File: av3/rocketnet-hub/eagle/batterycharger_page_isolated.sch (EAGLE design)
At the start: 45 parts, among them Q1 SIS412DNSOP-8, Q2 FDS6680ASOIC-8, Q3 FDS6680ASOIC-8, Q4 BSS138W-7-F, Q5 FDS6680ASOIC-8, Q6 SIS412DNSOP-8, U1 BQ24725QFN-20, U8 4.7uH

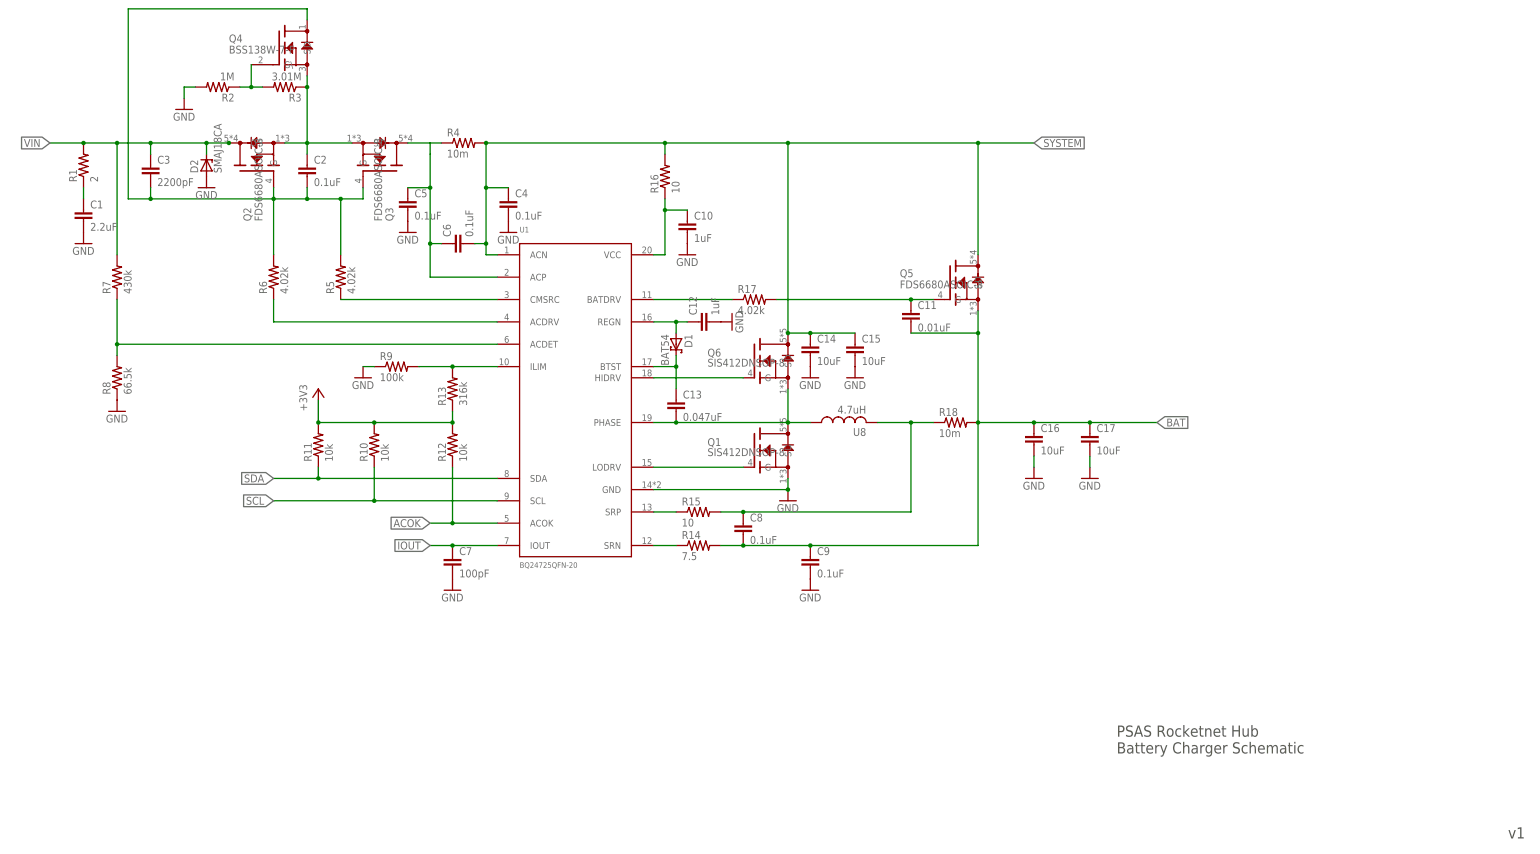
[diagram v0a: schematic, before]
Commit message: battery charger current state
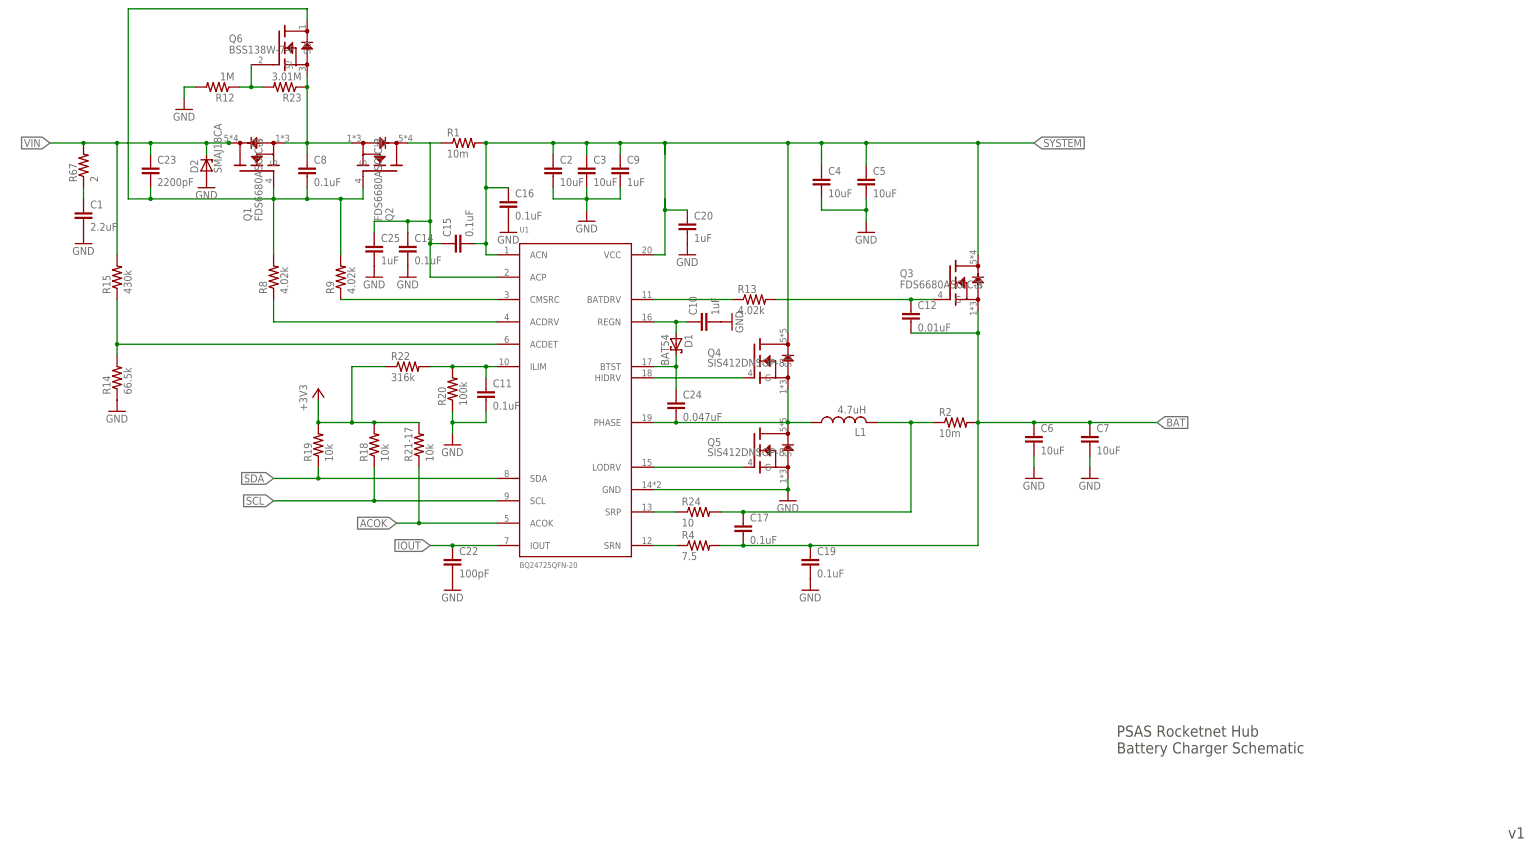
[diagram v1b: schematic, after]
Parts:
- removed C13: 0.047uF, rcl_custom:C-EU0603-B
- removed R10, R11: 10k, rcl_custom:R-US_R0603
- removed R16: 10, rcl_custom:R-US_1206-B
- removed R17, R5, R6: 4.02k, rcl_custom:R-US_0603-B
- removed R3: 3.01M, rcl_custom:R-US_0603-B
- removed R7: 430k, rcl_custom:R-US_0603-B
- added C19: 0.1uF, rcl_custom:C-EU0402-B
- added C20, C25: 1uF, rcl_custom:C-EU0603-B
- added C22: 100pF, rcl_custom:C-EU0402-B
- added C23: 2200pF, rcl_custom:C-EU0402-B
- added C24: 0.047uF, rcl_custom:C-EU0402-B
- added R19, R21-17: 10k, rcl_custom:R-US_0402-B
- added R20: 100k, rcl_custom:R-US_0402-B
- added R22: 316k, rcl_custom:R-US_0402-B
- added R23: 3.01M, rcl_custom:R-US_0402-B
- added R24: 10, rcl_custom:R-US_0603-B
- added R67: 2, rcl_custom:R-US_1206-B
- C11: value 0.01uF -> 0.1uF; device rcl_custom:C-EU0603-B -> rcl_custom:C-EU0402-B
- C12: value 1uF -> 0.01uF; device rcl_custom:C-EU0603-B -> rcl_custom:C-EU0402-B
- C14, C15, C16, C17: value 10uF -> 0.1uF; device rcl_custom:C-EU1206-B -> rcl_custom:C-EU0402-B
- C2, C4, C5, C6: value 0.1uF -> 10uF; device rcl_custom:C-EU0603-B -> rcl_custom:C-EU1206-B
- C3: value 2200pF -> 10uF; device rcl_custom:C-EU0603-B -> rcl_custom:C-EU1206-B
- C7: value 100pF -> 10uF; device rcl_custom:C-EUC0603 -> rcl_custom:C-EU1206-B
- C8: device rcl_custom:C-EU0603-B -> rcl_custom:C-EU0402-B
- C9: value 0.1uF -> 1uF
- Q1: value SIS412DNSOP-8 -> FDS6680ASOIC-8; device RNH_SIS412DN:SIS412DNSOP-8 -> RNH_FDS6680A:FDS6680ASOIC-8
- Q4: value BSS138W-7-F -> SIS412DNSOP-8; device RNH_BSS138W-7-F:BSS138W-7-F -> RNH_SIS412DN:SIS412DNSOP-8
- Q5: value FDS6680ASOIC-8 -> SIS412DNSOP-8; device RNH_FDS6680A:FDS6680ASOIC-8 -> RNH_SIS412DN:SIS412DNSOP-8
- Q6: value SIS412DNSOP-8 -> BSS138W-7-F; device RNH_SIS412DN:SIS412DNSOP-8 -> RNH_BSS138W-7-F:BSS138W-7-F
- R1: value 2 -> 10m
- R12: value 10k -> 1M; device rcl_custom:R-US_R0603 -> rcl_custom:R-US_0402-B
- R13: value 316k -> 4.02k; device rcl_custom:R-US_R0603 -> rcl_custom:R-US_0402-B
- R14: value 7.5 -> 66.5k; device rcl_custom:R-US_0603-B -> rcl_custom:R-US_0402-B
- R15: value 10 -> 430k; device rcl_custom:R-US_0603-B -> rcl_custom:R-US_0402-B
- R18: value 10m -> 10k; device rcl_custom:R-US_1206-B -> rcl_custom:R-US_0402-B
- R2: value 1M -> 10m; device rcl_custom:R-US_0603-B -> rcl_custom:R-US_1206-B
- R4: value 10m -> 7.5; device rcl_custom:R-US_1206-B -> rcl_custom:R-US_0603-B
- R8: value 66.5k -> 4.02k; device rcl_custom:R-US_1206-B -> rcl_custom:R-US_0402-B
- R9: value 100k -> 4.02k; device rcl_custom:R-US_R0603 -> rcl_custom:R-US_0402-B
- renumbered U8 to L1
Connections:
- removed net N$17: C10.1, R16.1, U1.VCC
- net +3V3: now also R18.2, R19.2, R21-17.2, R22.1; no longer R10.2, R11.2, R12.2, R13.1
- net ACOK: now also R21-17.1; no longer R12.1
- net BAT: now also C12.2, C17.2, C19.1, C6.1, C7.1, Q3.S, R2.2, R4.2; no longer C11.2, C16.1, C17.1, C8.2, C9.1, Q5.S, R14.2, R18.2
- net GND: now also C11.2, C19.2, C2.2, C20.2, C22.2, C25.2, C3.2, C6.2, Q5.S, R12.2, R14.1, R20.1; no longer C12.2, C15.2, C17.2, Q1.S, R2.2, R8.1, R9.1
- net IOUT: now also C22.1; no longer C7.1
- net N$1: now also C23.2, C8.2, Q1.G, Q6.D, R8.2, R9.2; no longer C2.2, C3.2, Q3.G, Q4.D, R5.2, R6.2
- net N$10: now also R14.2, R15.1; no longer R7.1, R8.2
- net N$11: now also C11.1, R20.2, R22.2; no longer R13.2, R9.2
- net N$12: now also R24.1; no longer R15.1
- net N$14: now also R4.1; no longer R14.1
- net N$15: now also C24.2, Q4.S, Q5.D; no longer C13.2, Q1.D, Q6.S
- net N$16: now also C17.1, R2.1, R24.2; no longer C8.1, R15.2, R18.1
- net N$18: now also R13.1; no longer R17.1
- net N$19: now also C12.1, Q3.G, R13.2; no longer C11.1, Q5.G, R17.2
- net N$2: now also Q6.G\, R12.1, R23.2; no longer Q4.G\, R2.1, R3.2
- net N$20: now also Q4.G; no longer Q6.G
- net N$21: now also C10.1; no longer C12.1
- net N$22: now also C24.1; no longer C13.1
- net N$25: now also Q5.G; no longer Q1.G
- net N$3: now also R67.1; no longer R1.1
- net N$5: now also C8.1, Q1.S, Q6.S, R23.1; no longer C2.1, Q3.S, Q4.S, R3.1
- net N$6: now also C14.1, C15.1, C25.1, Q2.D, R1.1; no longer C5.1, C6.1, Q3.D, R4.1
- net N$8: now also R9.1; no longer R5.1
- net N$9: now also R8.1; no longer R6.1
- net SCL: now also R18.1; no longer R10.1
- net SDA: now also R19.1; no longer R11.1
- net SYSTEM: now also C15.2, C16.1, C2.1, C20.1, C3.1, C5.1, C9.1, Q3.D, Q4.D, R1.2, U1.VCC; no longer C14.1, C15.1, C6.2, Q5.D, Q6.D, R16.2, R4.2
- net VIN: now also C23.1, Q1.D, R15.2, R67.2; no longer C3.1, Q2.D, R1.2, R7.2
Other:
- moved on the sheet: C10, C11, C12, C14, C15, C16, C17, C2, C3, C4, C5, C6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
